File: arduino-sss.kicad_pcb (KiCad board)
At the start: 2 copper layers, 68.6 x 53.3 mm, 47 parts, among them J1 Conn_01x03_Male, J2 Barrel_Jack_Switch, J3 DB9_Male, J4 Conn_01x02_Male, J5 Conn_02x03_Odd_Even, P1 Power, P2 Analog, P3 Digital, P4 Digital, P5 CONN_01X01, P6 CONN_01X01, P7 CONN_01X01, P8 CONN_01X01, Q1 BC547, Q2 BC557, SW1 SW_Push, U1 LM7805_TO220, U2 ATmega8-16PU, Y1 16000

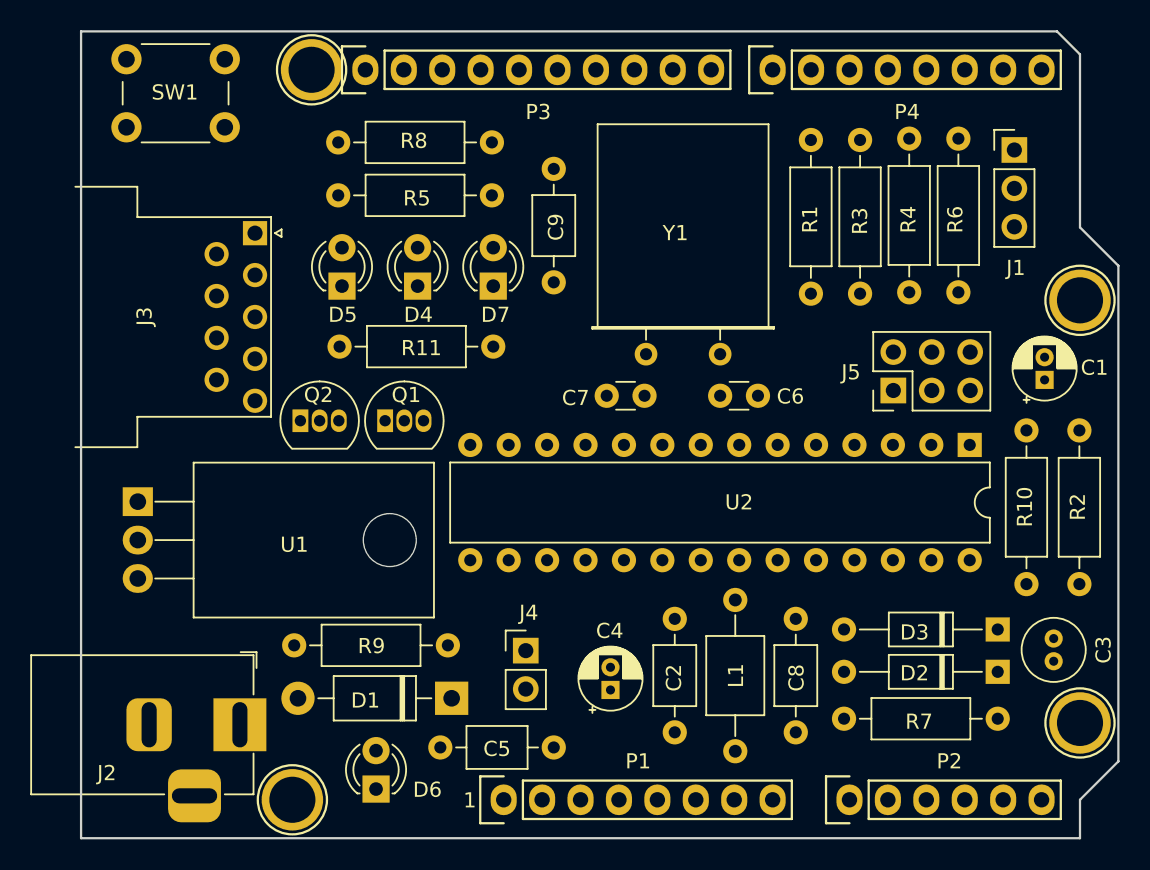
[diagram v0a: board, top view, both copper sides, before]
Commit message: update
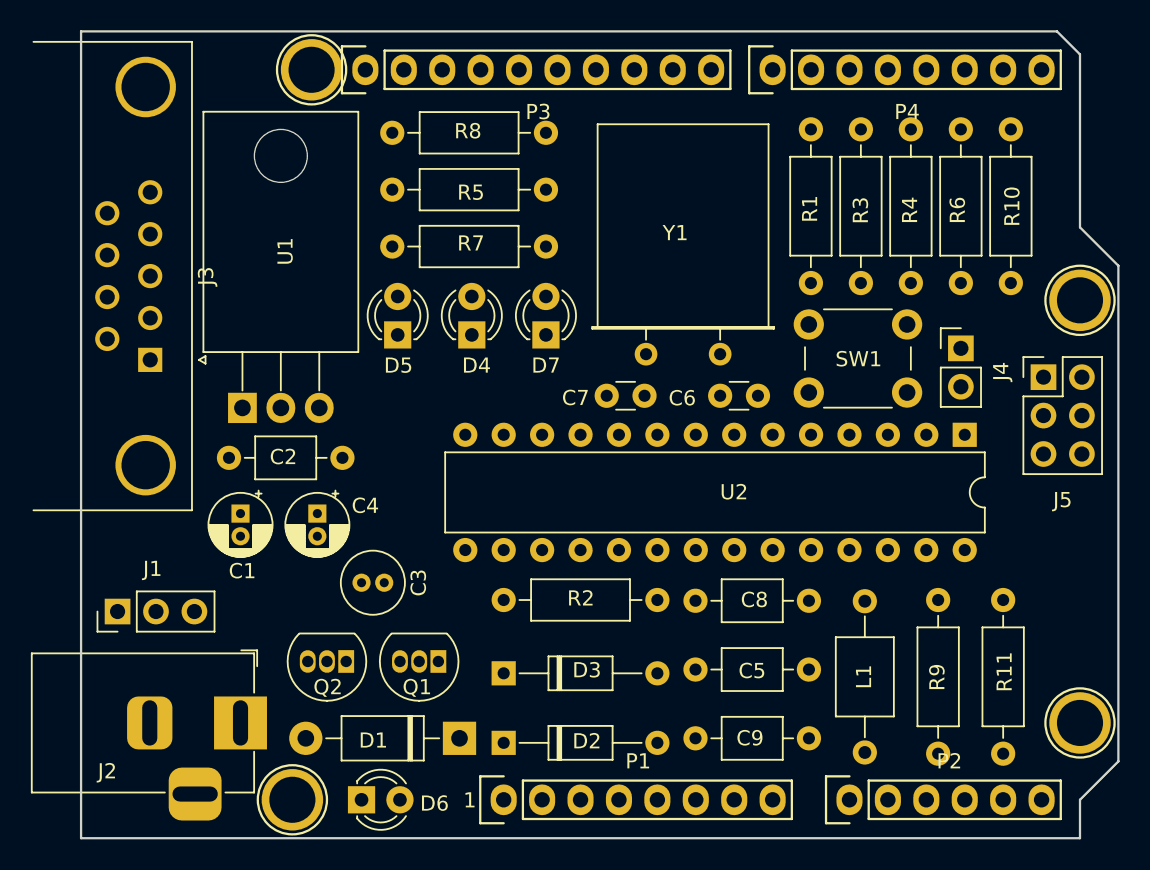
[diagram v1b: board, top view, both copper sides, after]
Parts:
- J3: value DB9_Male -> DB9_Female_MountingHoles; footprint Connector_Dsub:DSUB-9_Male_Horizontal_P2.77x2.54mm_EdgePinOffset9.40mm -> Connector_Dsub:DSUB-9_Female_Horizontal_P2.77x2.84mm_EdgePinOffset4.94mm_Housed_MountingHolesOffset7.48mm
- moved J1 66.7 mm to (113.4, 111.4), turned to 90 degrees
- moved SW1 56.1 mm to (165.6, 96.9), turned to 180 degrees
- moved C1 53.9 mm to (121.5, 104.9), turned to 270 degrees
- moved R7 50.8 mm to (131.6, 87.2), turned to 0 degrees
- moved C3 46.1 mm to (129.5, 109.5), turned to 0 degrees
- moved R9 42.7 mm to (167.7, 110.6), turned to 270 degrees
- moved C9 38.8 mm to (151.6, 119.8), turned to 0 degrees
- moved R2 38.1 mm to (138.9, 110.6), turned to 0 degrees
- moved R11 37.6 mm to (172.0, 110.6), turned to 270 degrees
- moved J4 35.0 mm to (169.2, 94.0)
- moved C2 34.6 mm to (120.8, 101.2), turned to 0 degrees
- moved D2 33.0 mm to (138.9, 120.1), turned to 0 degrees
- moved D3 32.8 mm to (138.9, 115.5), turned to 0 degrees
- moved R10 30.1 mm to (172.5, 79.5), turned to 270 degrees
- moved C4 22.6 mm to (126.6, 104.9), turned to 270 degrees
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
